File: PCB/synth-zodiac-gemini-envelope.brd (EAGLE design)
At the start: 76.1 x 72.4 mm, 28 parts, among them Q1 PNP, U1 TL074A

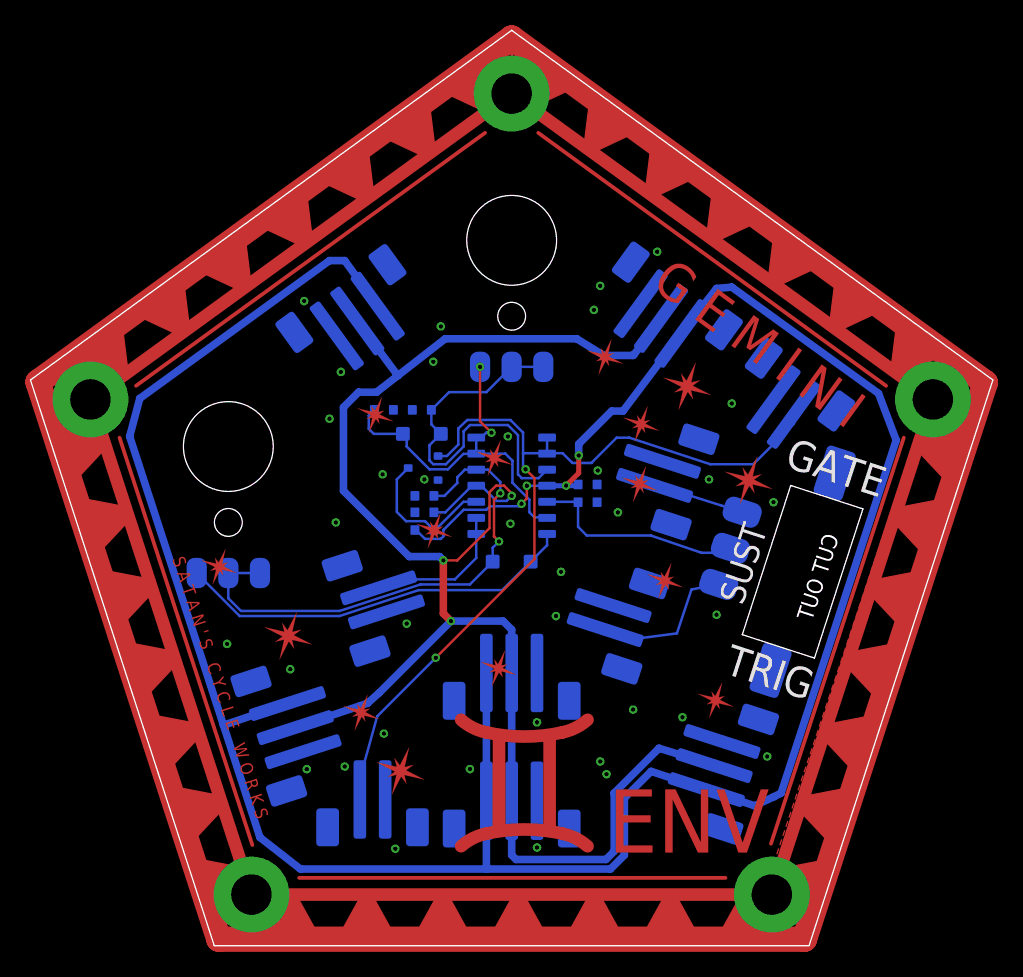
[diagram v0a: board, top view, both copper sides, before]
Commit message: Work in progress for rev A,  VCO rev.B
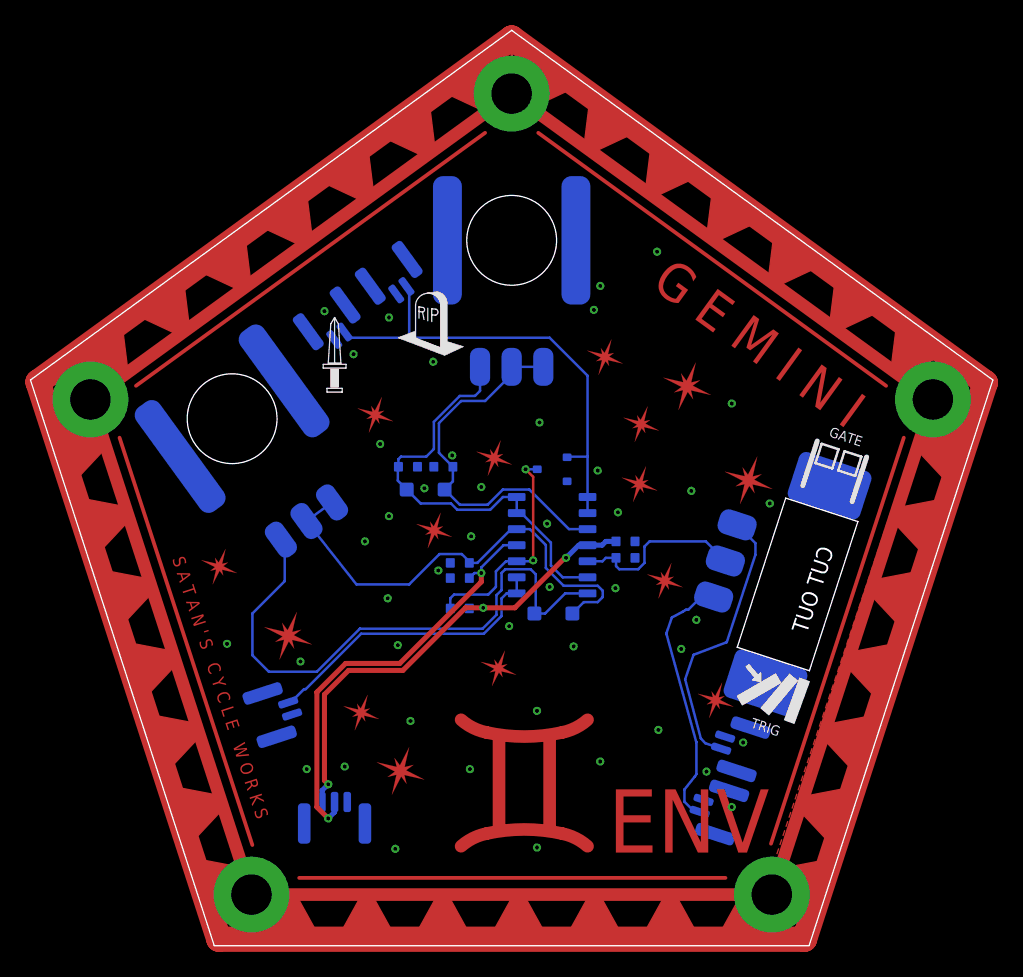
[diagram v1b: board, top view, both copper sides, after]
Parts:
- removed EG2VCF_MOD, EG2VCO_MOD: 2-pin, VT, SMT, con-jst:B2B-PH-SM4
- removed PWR_LFO, PWR_VCF, PWR_VCF_MOD, PWR_VCO, PWR_VCO_MOD: JST, 3P, VT, SMT, con-jst:B3B-PH-SM4
- removed SUST: SPDT, switch-thd:SS-12-F45-PNL-SMT
- added EG2VCFMOD, EG2VCOMOD: JST, SH, 2P, con-jst:BM02B-SRSS-TB
- added SRC: (no value), switch-thd:SS-12-F45-PNL-SMT
- EG2VCA, GATE_IN, TRIG_IN: value 2-pin, VT, SMT -> JST, SH, 2P; device con-jst:B2B-PH-SM4 -> con-jst:BM02B-SRSS-TB
- PWR_IN: value JST, 3P, VT, SMT -> JST SM 3P; device con-jst:B3B-PH-SM4 -> con-jst:BM03B-SRSS-TB
- moved GATE_IN 21.0 mm to (55.0, 16.6)
- moved PWR_IN 16.3 mm to (24.0, 11.7)
- moved TRIG_IN 15.3 mm to (53.3, 11.6)
- moved Q1 10.2 mm to (41.2, 38.3)
- moved EG2VCA 9.71 mm to (20.2, 19.3)
- moved R3 6.80 mm to (33.9, 27.3), turned to 180 degrees
- moved C1 5.99 mm to (33.9, 30.9)
- moved C4 5.91 mm to (33.9, 29.7)
- moved U1 5.69 mm to (41.2, 32.3)
- moved C3 5.41 mm to (47.0, 32.6)
- moved R1 5.33 mm to (47.0, 31.3)
- moved D1 5.26 mm to (41.3, 26.9), turned to 180 degrees
- moved R2 4.88 mm to (29.8, 38.5)
- moved C2 4.81 mm to (32.6, 38.5)
- moved D2 4.41 mm to (31.2, 36.7)
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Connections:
- net +9V: no longer PWR_LFO.1, PWR_VCF.1, PWR_VCF_MOD.1, PWR_VCO.1, PWR_VCO_MOD.1
- net -9V: no longer PWR_LFO.2, PWR_VCF.2, PWR_VCF_MOD.2, PWR_VCO.2, PWR_VCO_MOD.2
- net EG: now also EG2VCFMOD.1, EG2VCOMOD.1; no longer EG2VCF_MOD.1, EG2VCO_MOD.1
- net GATE: now also SRC.B; no longer SUST.B
- net GND: now also EG2VCFMOD.2, EG2VCOMOD.2, SRC.MTG1, SRC.MTG2; no longer EG2VCF_MOD.2, EG2VCO_MOD.2, PWR_LFO.3, PWR_VCF.3, PWR_VCF_MOD.3, PWR_VCO.3, PWR_VCO_MOD.3, SUST.MTG1, SUST.MTG2
- net N$134: now also SRC.C; no longer SUST.C
- net TRIG: now also SRC.A; no longer SUST.A
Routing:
- net +9V: track 215.2 -> 38.0 mm, vias 4 -> 3
- net -9V: track 134.7 -> 34.3 mm, vias 3 -> 2
- net EG: track 70.0 -> 37.3 mm, vias 2 -> 0
- net N$136: track 31.8 -> 46.5 mm
- net GATE: track 7.27 -> 21.8 mm
- net EG_VCA: track 11.9 -> 23.7 mm
- net TRIG: track 11.9 -> 20.7 mm
- net N$140: track 11.6 -> 17.7 mm, vias 0 -> 2
- net N$139: track 30.0 -> 34.4 mm, vias 2 -> 0
- net N$137: track 40.5 -> 37.3 mm, vias 2 -> 0
- net N$134: track 17.1 -> 14.1 mm
